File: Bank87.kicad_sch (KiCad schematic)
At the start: 1 part, among them U1 XCKU5P-FFVB676

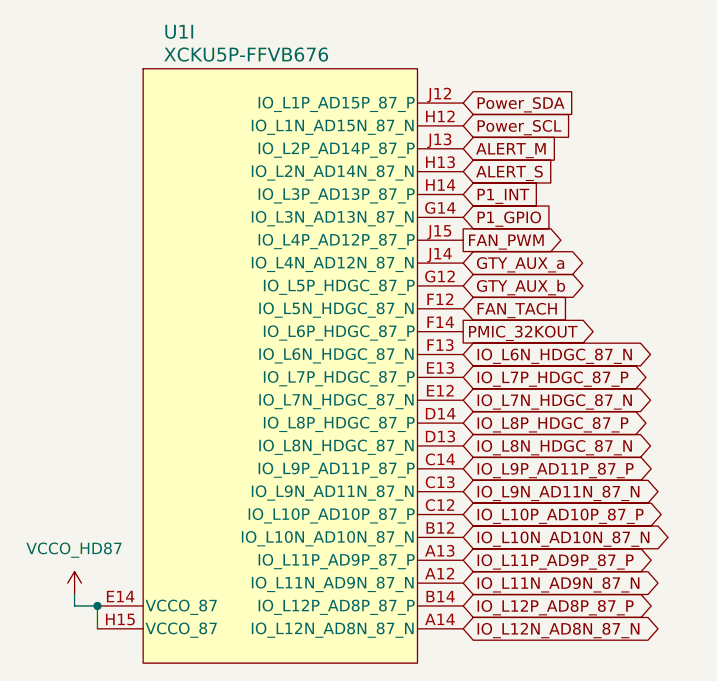
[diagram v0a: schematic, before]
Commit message: pushing the schematics works
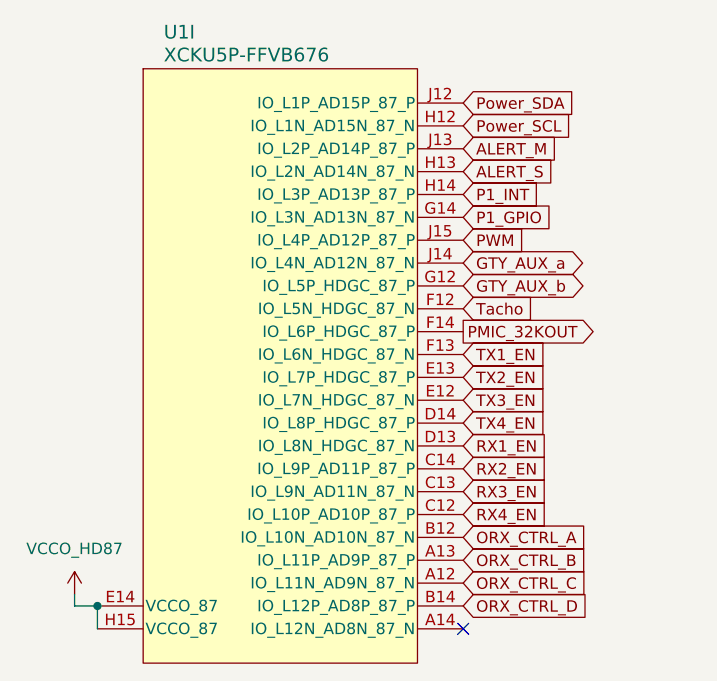
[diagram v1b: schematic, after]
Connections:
- net FAN_PWM renamed PWM
- net FAN_TACH renamed Tacho
- net IO_L10N_AD10N_87_N renamed ORX_CTRL_A
- net IO_L10P_AD10P_87_P renamed RX4_EN
- net IO_L11N_AD9N_87_N renamed ORX_CTRL_C
- net IO_L11P_AD9P_87_P renamed ORX_CTRL_B
- net IO_L12N_AD8N_87_N: no longer names the net of U1.A14 (IO_L12N_AD8N_87_N)
- net IO_L12P_AD8P_87_P renamed ORX_CTRL_D
- net IO_L6N_HDGC_87_N renamed TX1_EN
- net IO_L7N_HDGC_87_N renamed TX3_EN
- net IO_L7P_HDGC_87_P renamed TX2_EN
- net IO_L8N_HDGC_87_N renamed RX1_EN
- net IO_L8P_HDGC_87_P renamed TX4_EN
- net IO_L9N_AD11N_87_N renamed RX3_EN
- net IO_L9P_AD11P_87_P renamed RX2_EN
- no-connect marks 0 -> 1
